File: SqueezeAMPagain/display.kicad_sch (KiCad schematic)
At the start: 0 parts

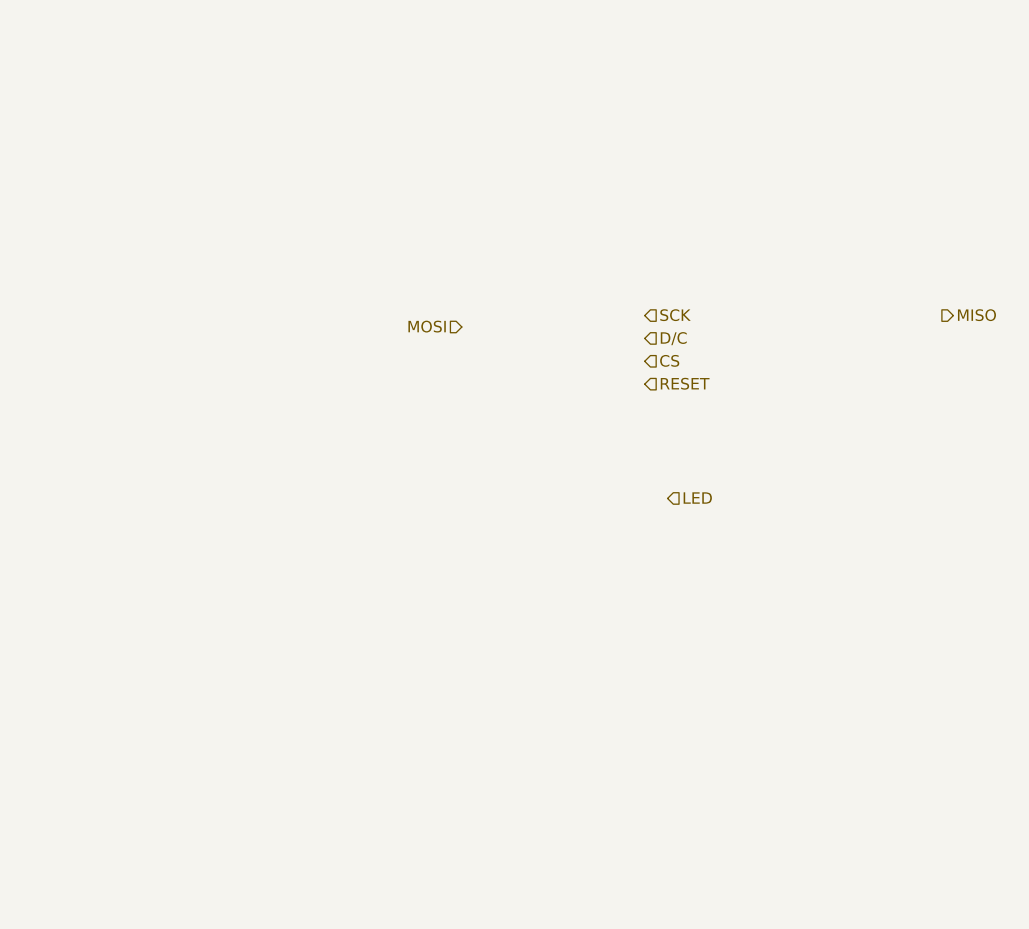
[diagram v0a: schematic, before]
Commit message: Update .gitignore, L_Radial_D12.0mm_P5+6+7.00mm_Fastron_11P.kicad_mod, SqueezeAMPagain.kicad_pcb, and 13 more files
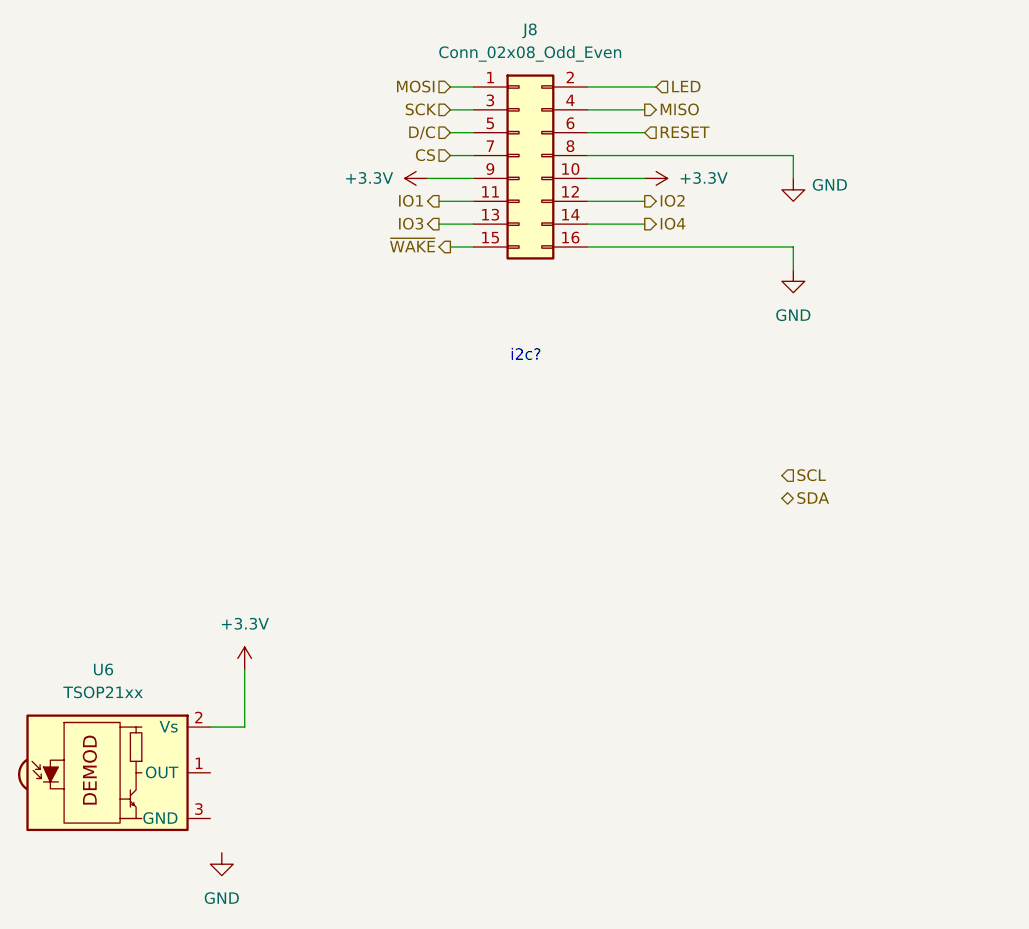
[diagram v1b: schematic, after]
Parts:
- added J8: Conn_02x08_Odd_Even, Connector_IDC:IDC-Header_2x08_P2.54mm_Vertical, symbol Connector_Generic:Conn_02x08_Odd_Even
- added U6: TSOP21xx, OptoDevice:Vishay_MOLD-3Pin, symbol Interface_Optical:TSOP21xx
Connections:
- net CS: now also J8.7 (Pin_7)
- net D/C: now also J8.5 (Pin_5)
- net LED: now also J8.2 (Pin_2)
- net MISO: now also J8.4 (Pin_4)
- net MOSI: now also J8.1 (Pin_1)
- net RESET: now also J8.6 (Pin_6)
- net SCK: now also J8.3 (Pin_3)
- new net +3.3V: J8.10 (Pin_10), J8.9 (Pin_9), U6.2 (Vs)
- new net GND: J8.16 (Pin_16), J8.8 (Pin_8)
- new net IO1: J8.11 (Pin_11)
- new net IO2: J8.12 (Pin_12)
- new net IO3: J8.13 (Pin_13)
- new net IO4: J8.14 (Pin_14)
- new net ~{WAKE}: J8.15 (Pin_15)
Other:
- note added: "i2c?"
- title: (none) -> Frontpanel connector
